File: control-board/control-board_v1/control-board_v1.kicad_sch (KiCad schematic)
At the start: 57 parts, among them J1 Barrel_Jack, J2 Header-M_2x6, J3 Header-M_2x6, J4 Header-M_2x6, J5 Header-M_2x6, J6 Header_1x8, J7 Header_1x8, J8 Header_1x10, J9 Header_1x8, Q1 PMOS, Q2 PMOS, Q3 PMOS, Q4 PMOS, Q5 PMOS, Q6 PMOS, Q7 PMOS, Q8 PMOS, U1 CD74HCT154M

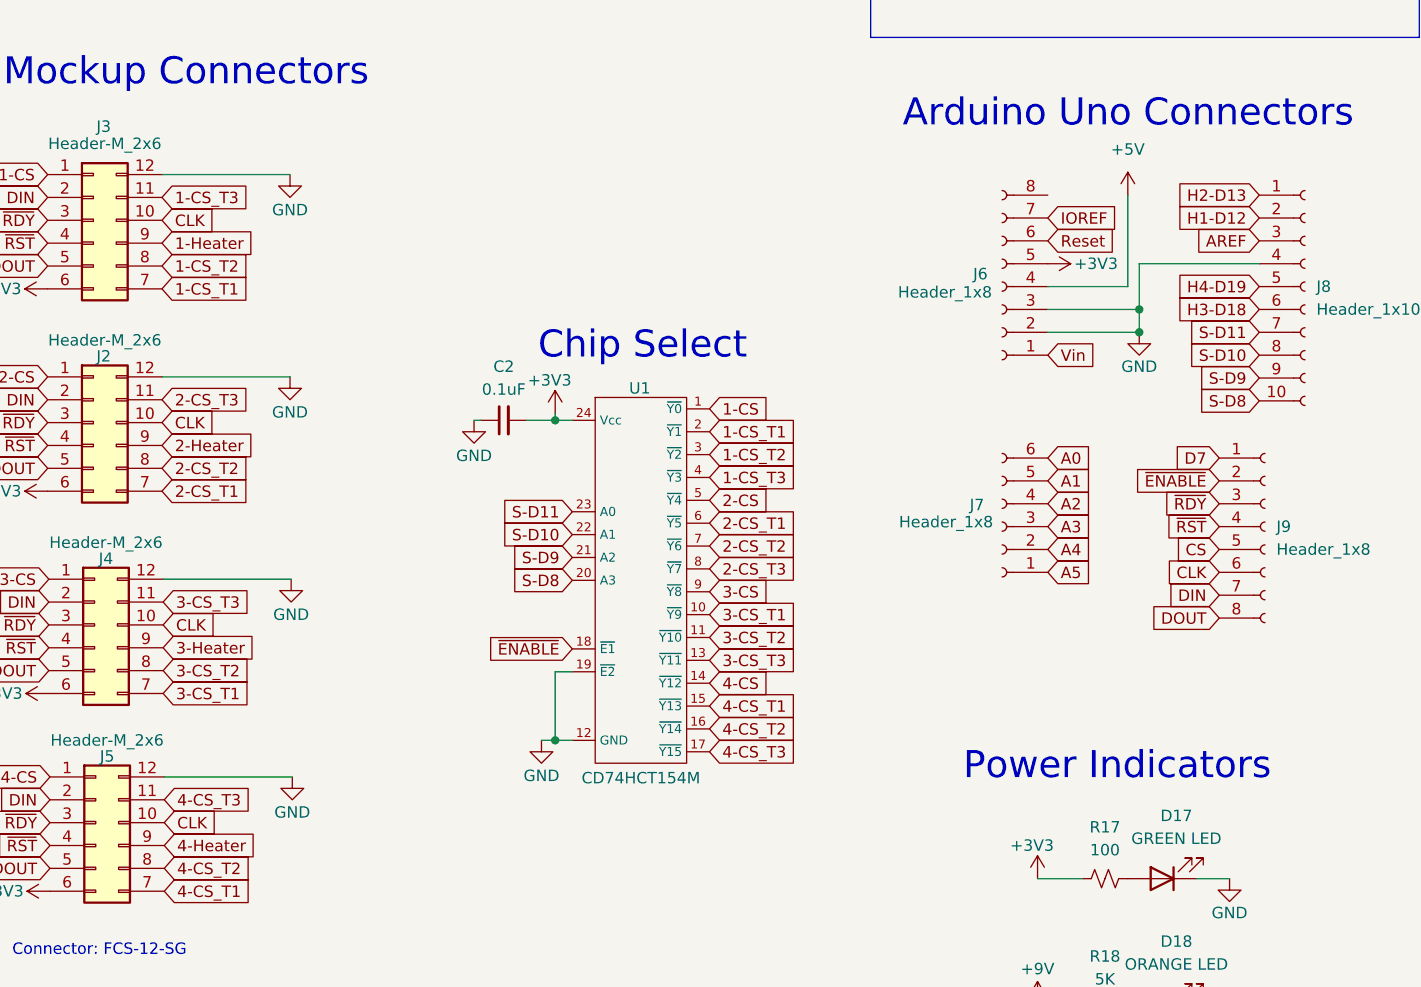
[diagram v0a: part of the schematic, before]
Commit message: pcb design change
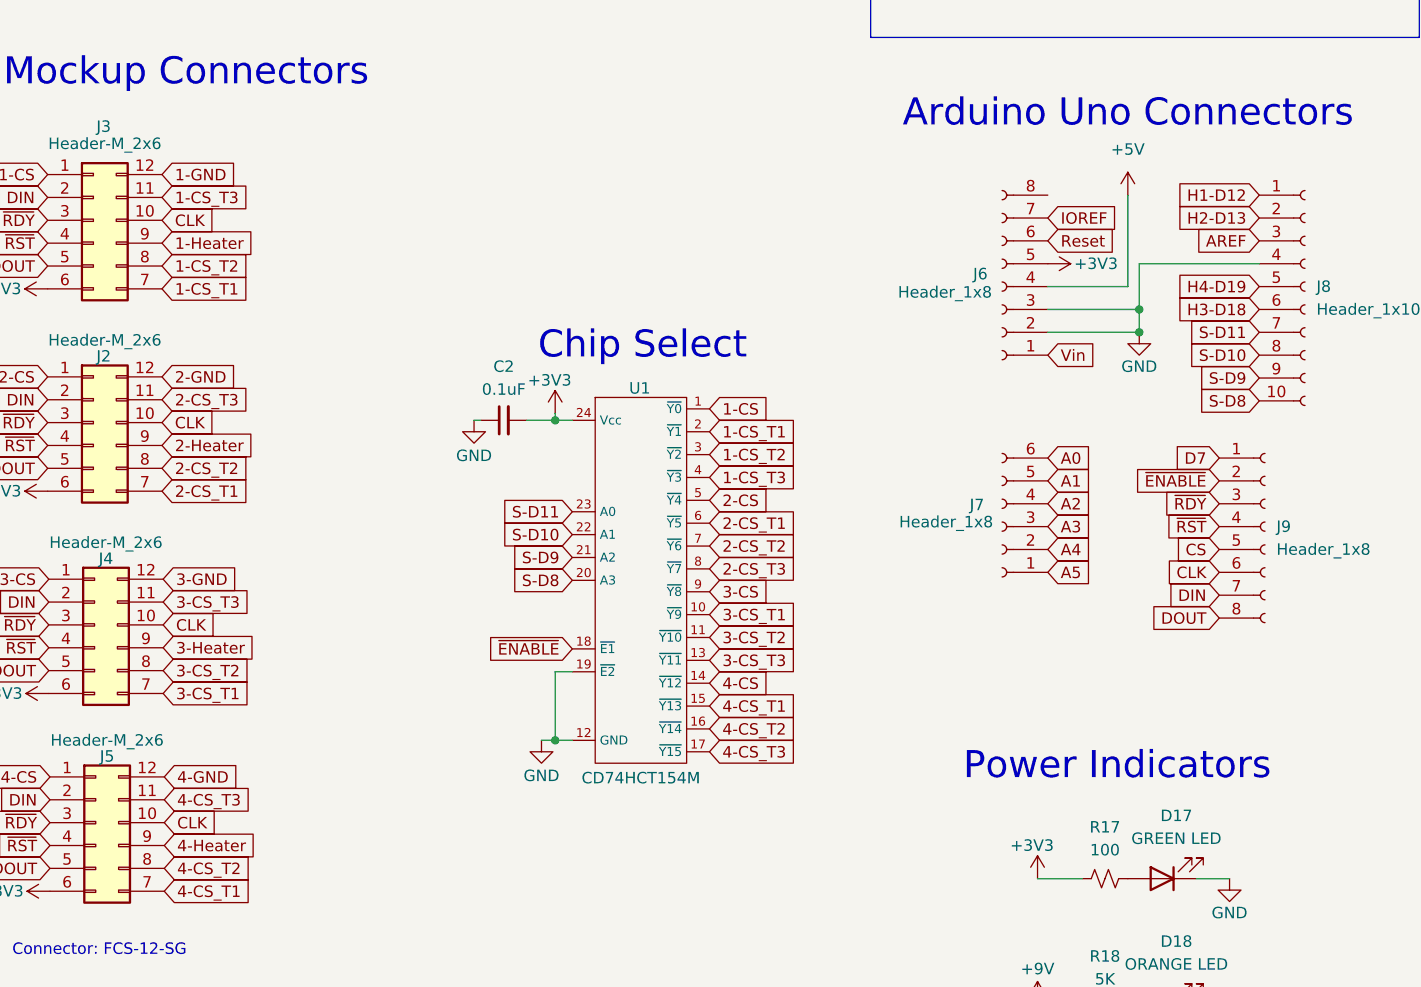
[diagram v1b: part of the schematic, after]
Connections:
- net GND: no longer J2.12 (Pin_12), J3.12 (Pin_12), J4.12 (Pin_12), J5.12 (Pin_12)
- net H1-D12: now also J8.1 (Pin_1); no longer J8.2 (Pin_2)
- net H2-D13: now also J8.2 (Pin_2); no longer J8.1 (Pin_1)
- new net 1-GND: J3.12 (Pin_12)
- new net 2-GND: J2.12 (Pin_12)
- new net 3-GND: J4.12 (Pin_12)
- new net 4-GND: J5.12 (Pin_12)
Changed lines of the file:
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@@
   )
   (no_connect (at 100.457 118.491))
-  (wire (pts (xy 158.115 109.601) (xy 143.891 109.601))
-    (stroke (width 0) (type default))
-  )
   (wire (pts (xy 179.197 91.948) (xy 178.435 91.948))
     (stroke (width 0) (type default))
@@
     (stroke (width 0) (type default))
   )
-  (wire (pts (xy 157.988 87.122) (xy 143.764 87.122))
-    (stroke (width 0) (type default))
-  )
   (wire (pts (xy 249.936 36.449) (xy 253.492 36.449))
     (stroke (width 0) (type default))
@@
     (stroke (width 0) (type default))
   )
-  (wire (pts (xy 157.988 64.643) (xy 143.764 64.643))
-    (stroke (width 0) (type default))
-  )
   (wire (pts (xy 187.452 91.948) (xy 189.357 91.948))
     (stroke (width 0) (type default))
@@
     (stroke (width 0) (type default))
   )
-  (wire (pts (xy 158.242 131.572) (xy 144.018 131.572))
-    (stroke (width 0) (type default))
-  )
   (wire (pts (xy 187.452 127.508) (xy 189.357 127.508))
     (stroke (width 0) (type default))
@@
     )
   )
-  (global_label "H2-D13" (shape input) (at 265.684 66.929 180) (fields_autoplaced)
-    (effects (font (size 1.27 1.27)) (justify right))
-    (property "Intersheetrefs" "${INTERSHEET_REFS}" (at 254.8974 66.929 0)
-      (effects (font (size 1.27 1.27)) (justify right) hide)
+  (global_label "1-GND" (shape input) (at 143.764 64.643 0) (fields_autoplaced)
+    (effects (font (size 1.27 1.27)) (justify left))
+    (property "Intersheetrefs" "${INTERSHEET_REFS}" (at 153.4016 64.643 0)
+      (effects (font (size 1.27 1.27)) (justify left) hide)
     )
   )
@@
     )
   )
+  (global_label "4-GND" (shape input) (at 144.018 131.572 0) (fields_autoplaced)
+    (effects (font (size 1.27 1.27)) (justify left))
+    (property "Intersheetrefs" "${INTERSHEET_REFS}" (at 153.6556 131.572 0)
+      (effects (font (size 1.27 1.27)) (justify left) hide)
+    )
+  )
   (global_label "1-CS" (shape input) (at 204.597 90.678 0) (fields_autoplaced)
     (effects (font (size 1.27 1.27)) (justify left))
@@
     )
   )
+  (global_label "H1-D12" (shape input) (at 265.684 66.929 180) (fields_autoplaced)
+    (effects (font (size 1.27 1.27)) (justify right))
+    (property "Intersheetrefs" "${INTERSHEET_REFS}" (at 254.8974 66.929 0)
+      (effects (font (size 1.27 1.27)) (justify right) hide)
+    )
+  )
   (global_label "S-D8" (shape input) (at 189.357 109.728 180) (fields_autoplaced)
     (effects (font (size 1.27 1.27)) (justify right))
@@
     )
   )
+  (global_label "H2-D13" (shape input) (at 265.684 69.469 180) (fields_autoplaced)
+    (effects (font (size 1.27 1.27)) (justify right))
+    (property "Intersheetrefs" "${INTERSHEET_REFS}" (at 254.8974 69.469 0)
+      (effects (font (size 1.27 1.27)) (justify right) hide)
+    )
+  )
   (global_label "CLK" (shape input) (at 261.239 108.839 180) (fields_autoplaced)
     (effects (font (size 1.27 1.27)) (justify right))
@@
     )
   )
+  (global_label "3-GND" (shape input) (at 143.891 109.601 0) (fields_autoplaced)
+    (effects (font (size 1.27 1.27)) (justify left))
+    (property "Intersheetrefs" "${INTERSHEET_REFS}" (at 153.5286 109.601 0)
+      (effects (font (size 1.27 1.27)) (justify left) hide)
+    )
+  )
   (global_label "1-CS_T2" (shape input) (at 143.764 74.803 0) (fields_autoplaced)
     (effects (font (size 1.27 1.27)) (justify left))
@@
     )
   )
-  (global_label "H1-D12" (shape input) (at 265.684 69.469 180) (fields_autoplaced)
-    (effects (font (size 1.27 1.27)) (justify right))
-    (property "Intersheetrefs" "${INTERSHEET_REFS}" (at 254.8974 69.469 0)
-      (effects (font (size 1.27 1.27)) (justify right) hide)
-    )
-  )
   (global_label "AREF" (shape input) (at 265.684 72.009 180) (fields_autoplaced)
     (effects (font (size 1.27 1.27)) (justify right))
@@
     )
   )
+  (global_label "2-GND" (shape input) (at 143.764 87.122 0) (fields_autoplaced)
+    (effects (font (size 1.27 1.27)) (justify left))
+    (property "Intersheetrefs" "${INTERSHEET_REFS}" (at 153.4016 87.122 0)
+      (effects (font (size 1.27 1.27)) (justify left) hide)
+    )
+  )
   (global_label "~{RDY}" (shape input) (at 131.064 92.202 180) (fields_autoplaced)
     (effects (font (size 1.27 1.27)) (justify right))
@@
     )
   )
-  (symbol (lib_id "power:GND") (at 158.115 109.601 0) (unit 1)
-    (in_bom yes) (on_board yes) (dnp no)
-    (property "Reference" "#PWR048" (at 158.115 115.951 0)
-      (effects (font (size 1.27 1.27)) hide)
-    )
-    (property "Value" "GND" (at 158.115 113.538 0)
-      (effects (font (size 1.27 1.27)))
-    )
-    (property "Footprint" "" (at 158.115 109.601 0)
-      (effects (font (size 1.27 1.27)) hide)
-    )
-    (property "Datasheet" "" (at 158.115 109.601 0)
-      (effects (font (size 1.27 1.27)) hide)
-    )
-    (pin "1")
-    (instances
-      (project "control-board_v1"
-        (path "/5ea0e920-d127-456d-9ad4-df9bbc649b9b"
-          (reference "#PWR048") (unit 1)
-        )
-      )
-    )
-  )
   (symbol (lib_id "Connector_Generic:Conn_02x06_Counter_Clockwise") (at 136.398 136.652 0) (unit 1)
     (in_bom yes) (on_board yes) (dnp no)
@@
     )
   )
-  (symbol (lib_id "power:GND") (at 157.988 87.122 0) (unit 1)
-    (in_bom yes) (on_board yes) (dnp no)
-    (property "Reference" "#PWR047" (at 157.988 93.472 0)
-      (effects (font (size 1.27 1.27)) hide)
-    )
-    (property "Value" "GND" (at 157.988 91.059 0)
-      (effects (font (size 1.27 1.27)))
-    )
-    (property "Footprint" "" (at 157.988 87.122 0)
-      (effects (font (size 1.27 1.27)) hide)
-    )
-    (property "Datasheet" "" (at 157.988 87.122 0)
-      (effects (font (size 1.27 1.27)) hide)
-    )
-    (pin "1")
-    (instances
-      (project "control-board_v1"
-        (path "/5ea0e920-d127-456d-9ad4-df9bbc649b9b"
-          (reference "#PWR047") (unit 1)
-        )
-      )
-    )
-  )
   (symbol (lib_id "power:+9V") (at 241.046 156.845 0) (unit 1)
     (in_bom yes) (on_board yes) (dnp no)
@@
     )
   )
-  (symbol (lib_id "power:GND") (at 157.988 64.643 0) (unit 1)
-    (in_bom yes) (on_board yes) (dnp no)
-    (property "Reference" "#PWR046" (at 157.988 70.993 0)
-      (effects (font (size 1.27 1.27)) hide)
-    )
-    (property "Value" "GND" (at 157.988 68.58 0)
-      (effects (font (size 1.27 1.27)))
-    )
-    (property "Footprint" "" (at 157.988 64.643 0)
-      (effects (font (size 1.27 1.27)) hide)
-    )
-    (property "Datasheet" "" (at 157.988 64.643 0)
-      (effects (font (size 1.27 1.27)) hide)
-    )
-    (pin "1")
-    (instances
-      (project "control-board_v1"
-        (path "/5ea0e920-d127-456d-9ad4-df9bbc649b9b"
-          (reference "#PWR046") (unit 1)
-        )
-      )
-    )
-  )
   (symbol (lib_id "Device:LED") (at 42.799 119.253 90) (unit 1)
     (in_bom yes) (on_board yes) (dnp no) (fields_autoplaced)
@@
         )
       )
-    )
-  )
-  (symbol (lib_id "power:GND") (at 158.242 131.572 0) (unit 1)
-    (in_bom yes) (on_board yes) (dnp no)
-    (property "Reference" "#PWR049" (at 158.242 137.922 0)
-      (effects (font (size 1.27 1.27)) hide)
-    )
-    (property "Value" "GND" (at 158.242 135.509 0)
-      (effects (font (size 1.27 1.27)))
-    )
-    (property "Footprint" "" (at 158.242 131.572 0)
-      (effects (font (size 1.27 1.27)) hide)
-    )
-    (property "Datasheet" "" (at 158.242 131.572 0)
-      (effects (font (size 1.27 1.27)) hide)
-    )
-    (pin "1")
-    (instances
-      (project "control-board_v1"
-        (path "/5ea0e920-d127-456d-9ad4-df9bbc649b9b"
-          (reference "#PWR049") (unit 1)
-        )
-      )
